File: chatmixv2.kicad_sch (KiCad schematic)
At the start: 16 parts, among them J1 USB_C_Receptacle_USB2.0_16P, U1 STM32F072RBTx, U2 AP2112K-3.3

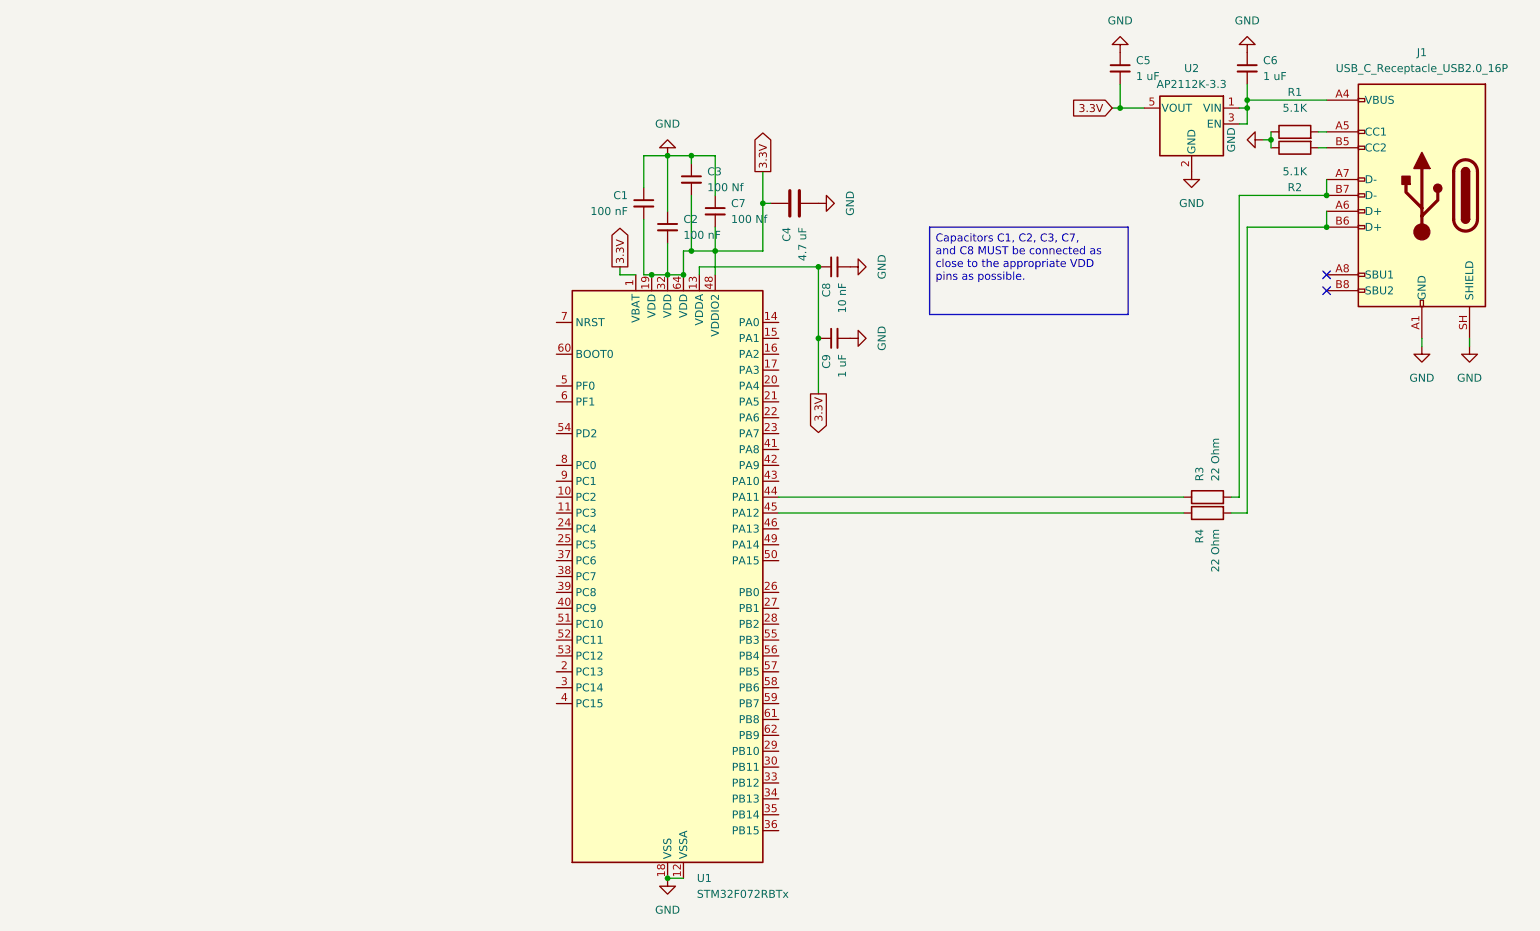
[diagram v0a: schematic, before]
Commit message: GPIO and fixes
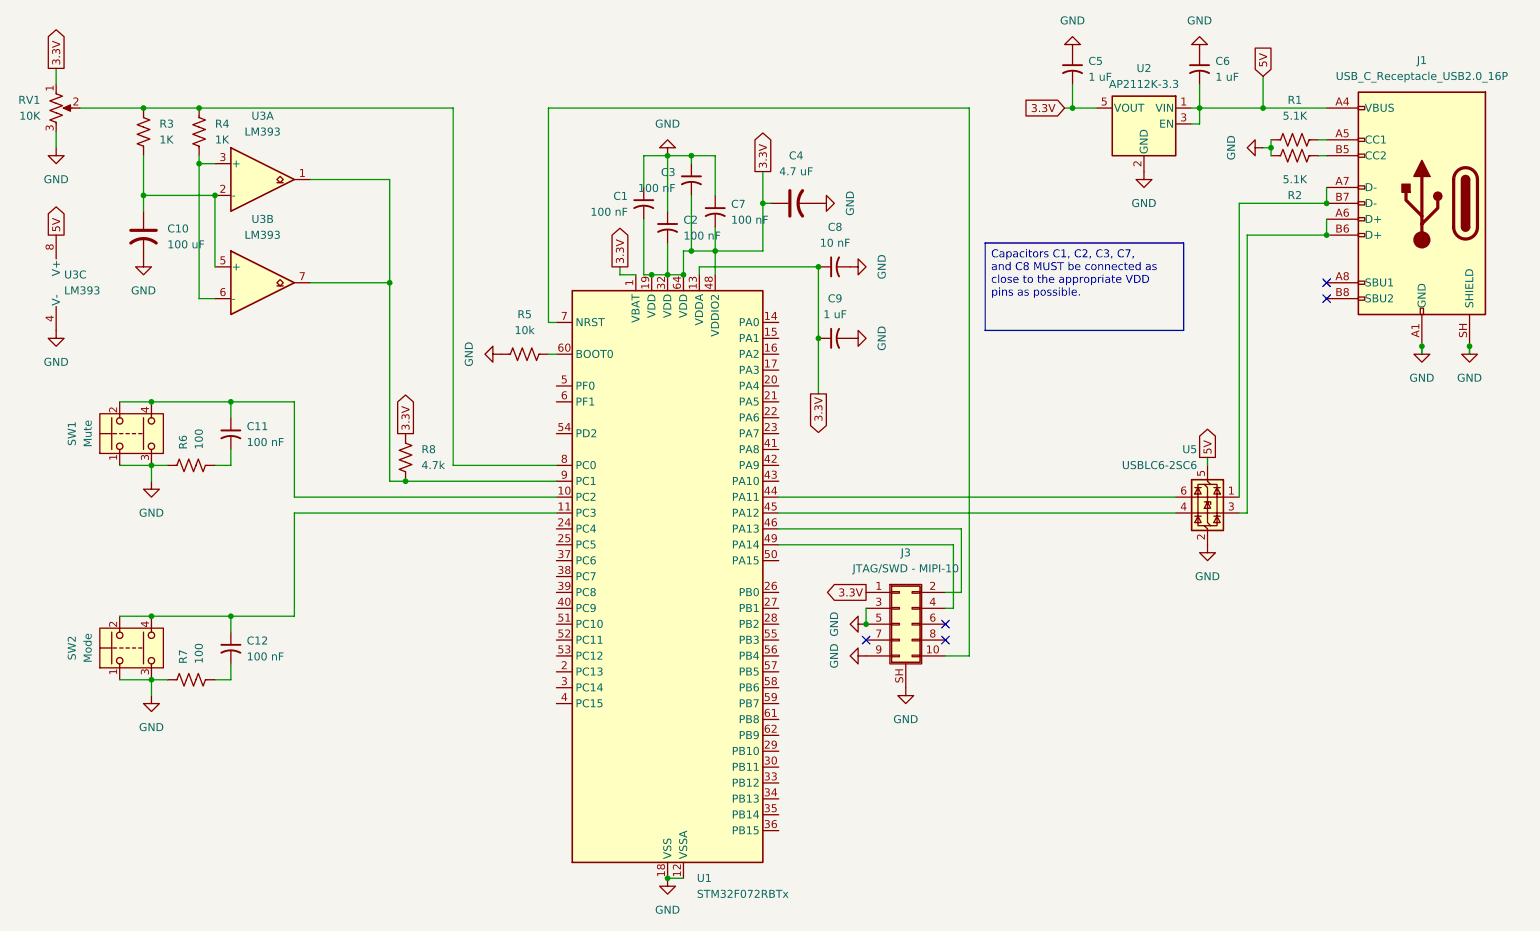
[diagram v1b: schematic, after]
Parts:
- removed R3, R4: 22 Ohm, symbol Device:R
- added C10: 100 uF, symbol Device:C_US
- added C11, C12: 100 nF, symbol Device:C_Small_US
- added J3: JTAG/SWD - MIPI-10, symbol Connector_Generic_Shielded:Conn_02x05_Odd_Even_Shielded
- added R3, R4: 1K, symbol Device:R_US
- added R5: 10k, symbol Device:R_US
- added R6, R7: 100, symbol Device:R_US
- added R8: 4.7k, symbol Device:R_US
- added RV1: 10K, symbol Device:R_Potentiometer_US
- added SW1: Mute, symbol Switch:SW_Push_Dual
- added SW2: Mode, symbol Switch:SW_Push_Dual
- added U3: LM393, symbol Comparator:LM393
- added U5: USBLC6-2SC6, Package_TO_SOT_SMD:SOT-23-6, symbol Power_Protection:USBLC6-2SC6
- C1, C2, C5, C6, C8, C9: symbol Device:C_Small -> Device:C_Small_US
- C3, C7: value 100 Nf -> 100 nF; symbol Device:C_Small -> Device:C_Small_US
- C4: symbol Device:C -> Device:C_US
- R1, R2: symbol Device:R -> Device:R_US
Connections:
- net 3.3V: now also J3.1 (Pin_1), R8.1, RV1.1
- net GND: now also C10.2, J3.3 (Pin_3), J3.5 (Pin_5), J3.9 (Pin_9), J3.SH (Shield), R5.1, R6.1, R7.1, RV1.3, SW1.1, SW1.3, SW2.1, SW2.3, U3.4 (V-), U5.2 (GND)
- net 5V: now reaches C6.2, J1.A4 (VBUS), J1.A9 (VBUS), J1.B4 (VBUS), J1.B9 (VBUS), U2.1 (VIN), U2.3 (EN)
- net 5V: now also U3.8 (V+), U5.5 (VBUS)
- net at J1.A6 (D+), J1.B6 (D+): now also U5.3 (I/O2)
- net at J1.A7 (D-), J1.B7 (D-): now also U5.1 (I/O1)
- net at U1.45 (PA12): now also U5.4 (I/O2)
- net at U1.10 (PC2): now also C11.1, SW1.2, SW1.4
- net at U1.11 (PC3): now also C12.1, SW2.2, SW2.4
- net at U1.44 (PA11): now also U5.6 (I/O1)
- net at U1.46 (PA13): now also J3.2 (Pin_2)
- net at U1.49 (PA14): now also J3.4 (Pin_4)
- net at U1.60 (BOOT0): now also R5.2
- net at U1.7 (NRST): now also J3.10 (Pin_10)
- net at U1.8 (PC0): now also R3.1, R4.1, RV1.2
- net at U1.9 (PC1): now also R8.2, U3.1, U3.7
- new net: R4.2, U3.3 (+), U3.6 (-)
- new net: C12.2, R7.2
- new net: C11.2, R6.2
- new net: C10.1, R3.2, U3.2 (-), U3.5 (+)
- no-connect marks 2 -> 5
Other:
- moved on the sheet: C5, C6, J1, U2
